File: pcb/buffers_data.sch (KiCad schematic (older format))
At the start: 8 parts, among them U1 74LVCH162245A, U2 74LVCH162245A

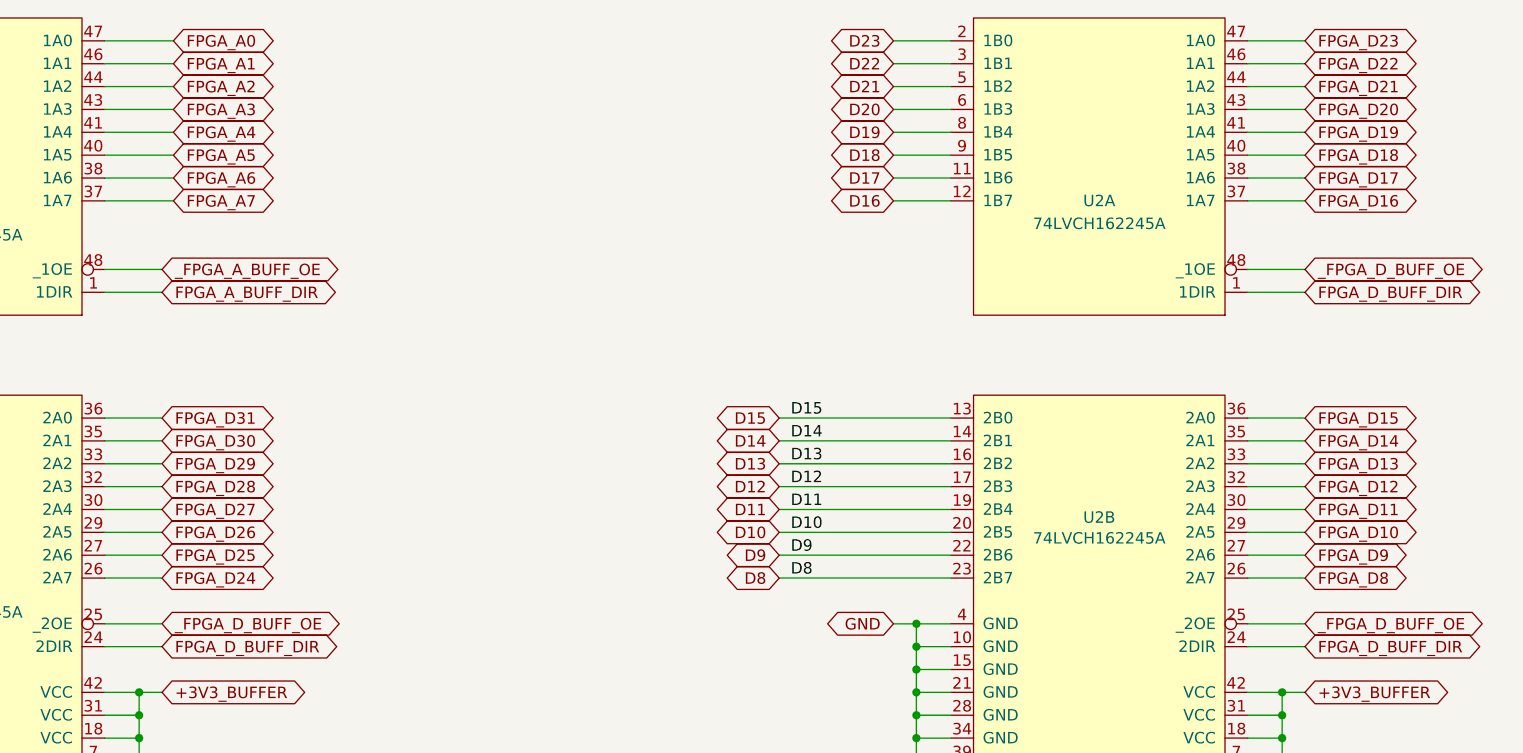
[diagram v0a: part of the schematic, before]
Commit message: some more work done
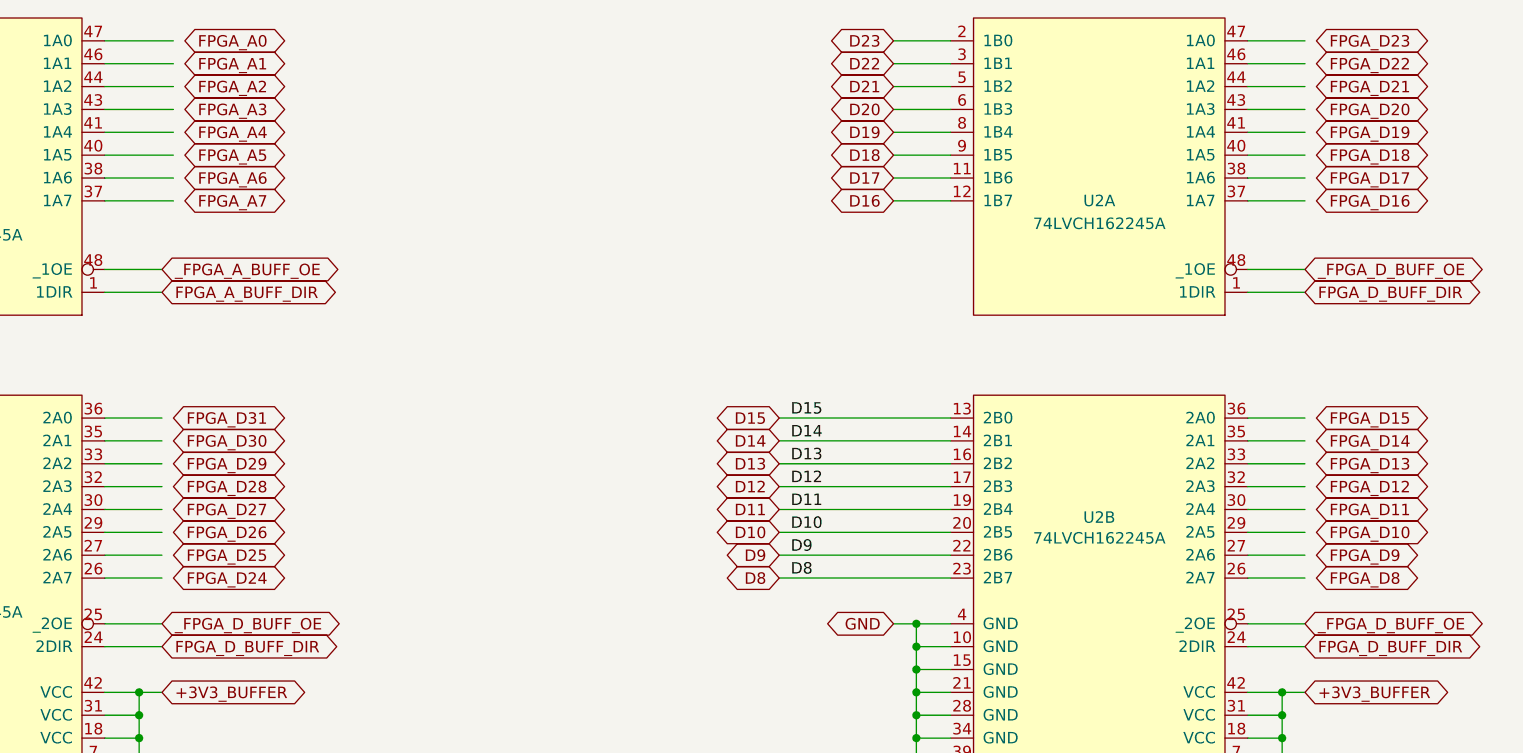
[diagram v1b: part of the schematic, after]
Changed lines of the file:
@@
 Text GLabel 9150 4200 2    50   BiDi ~ 0
 FPGA_D_BUFF_DIR
-Text GLabel 9150 1550 2    50   BiDi ~ 0
+Text GLabel 9200 1550 2    50   BiDi ~ 0
 FPGA_D23
-Text GLabel 9150 1650 2    50   BiDi ~ 0
+Text GLabel 9200 1650 2    50   BiDi ~ 0
 FPGA_D22
-Text GLabel 9150 1750 2    50   BiDi ~ 0
+Text GLabel 9200 1750 2    50   BiDi ~ 0
 FPGA_D21
-Text GLabel 9150 1850 2    50   BiDi ~ 0
+Text GLabel 9200 1850 2    50   BiDi ~ 0
 FPGA_D20
-Text GLabel 9150 1950 2    50   BiDi ~ 0
+Text GLabel 9200 1950 2    50   BiDi ~ 0
 FPGA_D19
-Text GLabel 9150 2050 2    50   BiDi ~ 0
+Text GLabel 9200 2050 2    50   BiDi ~ 0
 FPGA_D18
-Text GLabel 9150 2150 2    50   BiDi ~ 0
+Text GLabel 9200 2150 2    50   BiDi ~ 0
 FPGA_D17
-Text GLabel 9150 2250 2    50   BiDi ~ 0
+Text GLabel 9200 2250 2    50   BiDi ~ 0
 FPGA_D16
-Text GLabel 9150 3200 2    50   BiDi ~ 0
+Text GLabel 9200 3200 2    50   BiDi ~ 0
 FPGA_D15
-Text GLabel 9150 3300 2    50   BiDi ~ 0
+Text GLabel 9200 3300 2    50   BiDi ~ 0
 FPGA_D14
-Text GLabel 9150 3400 2    50   BiDi ~ 0
+Text GLabel 9200 3400 2    50   BiDi ~ 0
 FPGA_D13
-Text GLabel 9150 3500 2    50   BiDi ~ 0
+Text GLabel 9200 3500 2    50   BiDi ~ 0
 FPGA_D12
-Text GLabel 9150 3600 2    50   BiDi ~ 0
+Text GLabel 9200 3600 2    50   BiDi ~ 0
 FPGA_D11
-Text GLabel 9150 3700 2    50   BiDi ~ 0
+Text GLabel 9200 3700 2    50   BiDi ~ 0
 FPGA_D10
-Text GLabel 9150 3800 2    50   BiDi ~ 0
+Text GLabel 9200 3800 2    50   BiDi ~ 0
 FPGA_D9
-Text GLabel 9150 3900 2    50   BiDi ~ 0
+Text GLabel 9200 3900 2    50   BiDi ~ 0
 FPGA_D8
 Wire Wire Line
@@
 Wire Wire Line
 	4150 4100 3900 4100
-Text GLabel 4150 3900 2    50   BiDi ~ 0
+Text GLabel 4200 3900 2    50   BiDi ~ 0
 FPGA_D24
-Text GLabel 4150 3800 2    50   BiDi ~ 0
+Text GLabel 4200 3800 2    50   BiDi ~ 0
 FPGA_D25
-Text GLabel 4150 3700 2    50   BiDi ~ 0
+Text GLabel 4200 3700 2    50   BiDi ~ 0
 FPGA_D26
-Text GLabel 4150 3600 2    50   BiDi ~ 0
+Text GLabel 4200 3600 2    50   BiDi ~ 0
 FPGA_D27
-Text GLabel 4150 3500 2    50   BiDi ~ 0
+Text GLabel 4200 3500 2    50   BiDi ~ 0
 FPGA_D28
-Text GLabel 4150 3400 2    50   BiDi ~ 0
+Text GLabel 4200 3400 2    50   BiDi ~ 0
 FPGA_D29
-Text GLabel 4150 3300 2    50   BiDi ~ 0
+Text GLabel 4200 3300 2    50   BiDi ~ 0
 FPGA_D30
-Text GLabel 4150 3200 2    50   BiDi ~ 0
+Text GLabel 4200 3200 2    50   BiDi ~ 0
 FPGA_D31
 Text GLabel 4150 4200 2    50   BiDi ~ 0
@@
 Wire Wire Line
 	3900 3200 4150 3200
-Text GLabel 4200 1550 2    50   BiDi ~ 0
+Text GLabel 4250 1550 2    50   BiDi ~ 0
 FPGA_A0
-Text GLabel 4200 1650 2    50   BiDi ~ 0
+Text GLabel 4250 1650 2    50   BiDi ~ 0
 FPGA_A1
-Text GLabel 4200 1750 2    50   BiDi ~ 0
+Text GLabel 4250 1750 2    50   BiDi ~ 0
 FPGA_A2
-Text GLabel 4200 1850 2    50   BiDi ~ 0
+Text GLabel 4250 1850 2    50   BiDi ~ 0
 FPGA_A3
-Text GLabel 4200 1950 2    50   BiDi ~ 0
+Text GLabel 4250 1950 2    50   BiDi ~ 0
 FPGA_A4
-Text GLabel 4200 2050 2    50   BiDi ~ 0
+Text GLabel 4250 2050 2    50   BiDi ~ 0
 FPGA_A5
-Text GLabel 4200 2150 2    50   BiDi ~ 0
+Text GLabel 4250 2150 2    50   BiDi ~ 0
 FPGA_A6
-Text GLabel 4200 2250 2    50   BiDi ~ 0
+Text GLabel 4250 2250 2    50   BiDi ~ 0
 FPGA_A7
 Wire Wire Line
